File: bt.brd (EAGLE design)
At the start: 24.4 x 17.8 mm, 16 parts, among them IC1 BLUETOOTH-RN42 HID, Q1 MOSFET-NCHANNELSMD, Q2 MOSFET-NCHANNELSMD

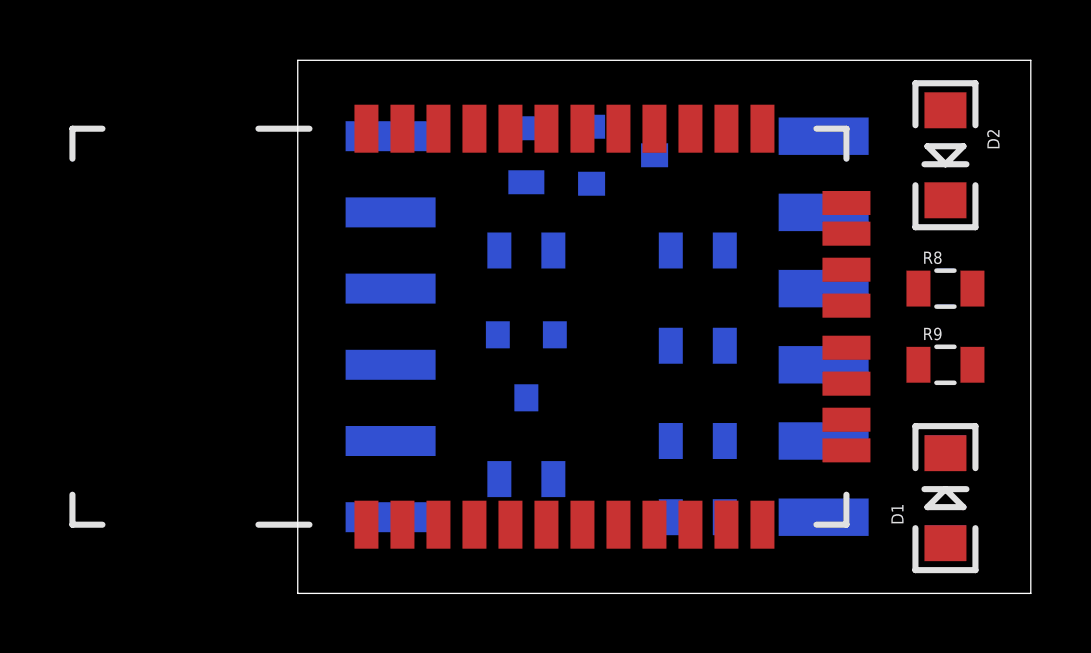
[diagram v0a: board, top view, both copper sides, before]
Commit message: Flipped the board around
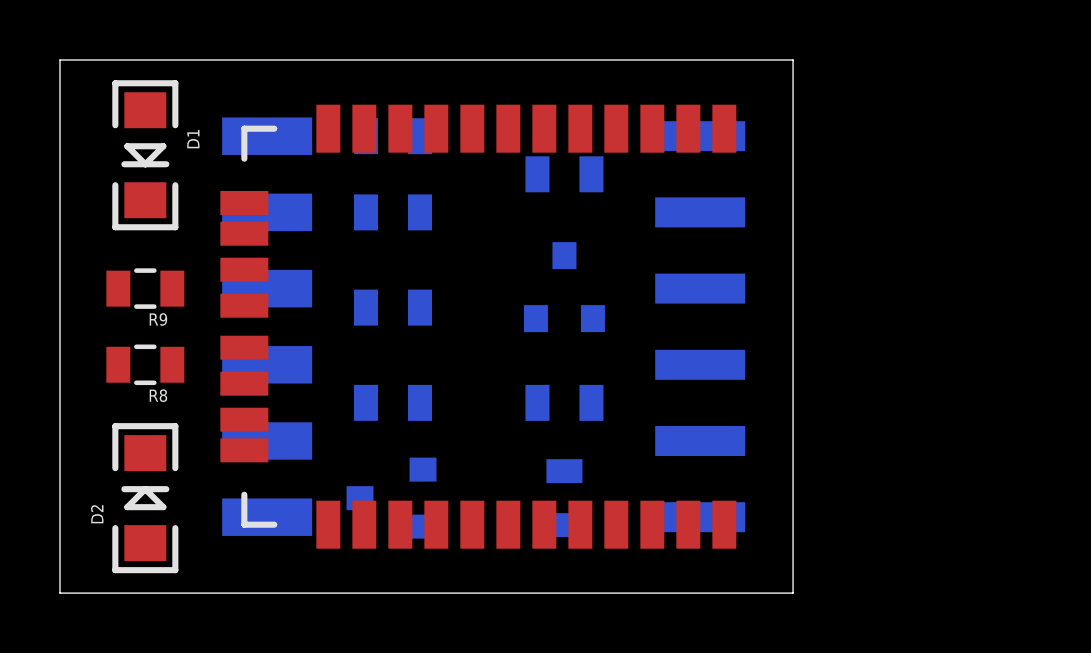
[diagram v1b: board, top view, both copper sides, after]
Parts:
- removed IC1: BLUETOOTH-RN42 HID, SparkFun-RF:RN41
- removed JP1: (no value), mine:1X06-SMD-FEMALE-V2-NOSILK
- removed JP2: RA 6Pin SMD, mine:1X06-SMD-NOHOLES
- added RN-42HID: BLUETOOTH-RN42-NOSILK", mine:RN41
- added UART: RA 6Pin SMD, mine:1X06-SMD-NOHOLES
- added USB: (no value), mine:1X06-SMD-FEMALE-V2-NOSILK
- moved D1 29.0 mm to (3.17, 14.6), turned to 270 degrees
- moved D2 29.0 mm to (3.17, 3.17), turned to 90 degrees
- moved R8 26.8 mm to (3.17, 7.62), turned to 180 degrees
- moved R9 26.8 mm to (3.17, 10.2), turned to 180 degrees
- moved R2 16.3 mm to (11.4, 15.2), turned to 0 degrees
- moved Q2 13.7 mm to (11.4, 3.17), turned to 270 degrees
- moved R7 12.7 mm to (11.4, 12.7), turned to 180 degrees
- moved R5 11.5 mm to (17.1, 3.17), turned to 90 degrees
- moved R6 11.4 mm to (11.4, 6.35), turned to 0 degrees
- moved R1 10.2 mm to (11.4, 9.53), turned to 0 degrees
- moved R4 10.2 mm to (17.1, 14.0), turned to 0 degrees
- moved R3 5.24 mm to (17.1, 6.35), turned to 180 degrees
- moved Q1 2.84 mm to (17.1, 10.2), turned to 0 degrees
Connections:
- net 3.3V: now also USB.6; no longer JP1.6
- net GND: now also RN-42HID.1, RN-42HID.12, RN-42HID.28, RN-42HID.29, UART.1, USB.1; no longer IC1.1, IC1.12, IC1.28, IC1.29, JP1.1, JP2.1
- net N$10: now also RN-42HID.21; no longer IC1.21
- net N$8: now also RN-42HID.19; no longer IC1.19
- net N$9: now also RN-42HID.22; no longer IC1.22
- net UART_CTS: now also RN-42HID.16; no longer IC1.16
- net UART_CTS_5V: now also UART.5; no longer JP2.5
- net UART_RTS: now also RN-42HID.15; no longer IC1.15
- net UART_RTS_5V: now also UART.2; no longer JP2.2
- net UART_RX: now also RN-42HID.13; no longer IC1.13
- net UART_RX_5V: now also UART.3; no longer JP2.3
- net UART_TX: now also RN-42HID.14; no longer IC1.14
- net UART_TX_5V: now also UART.4; no longer JP2.4
- net USB_D+: now also RN-42HID.17, USB.4; no longer IC1.17, JP1.4
- net USB_D-: now also RN-42HID.18, USB.3; no longer IC1.18, JP1.3
- net VCC: now also RN-42HID.11, UART.6, USB.5; no longer IC1.11, JP1.5, JP2.6
